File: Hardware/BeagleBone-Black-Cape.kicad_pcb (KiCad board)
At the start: 2 copper layers, 54.6 x 86.4 mm, 17 parts, among them J1 MISC, J2 POWER, J3 BOOT, J4 BOOT, M1 MR1132, M2 CC2538MODULE, P8 BeagleBone_Black_Header, P9 BeagleBone_Black_Header, Q1 2N7002, U1 MAX3072E

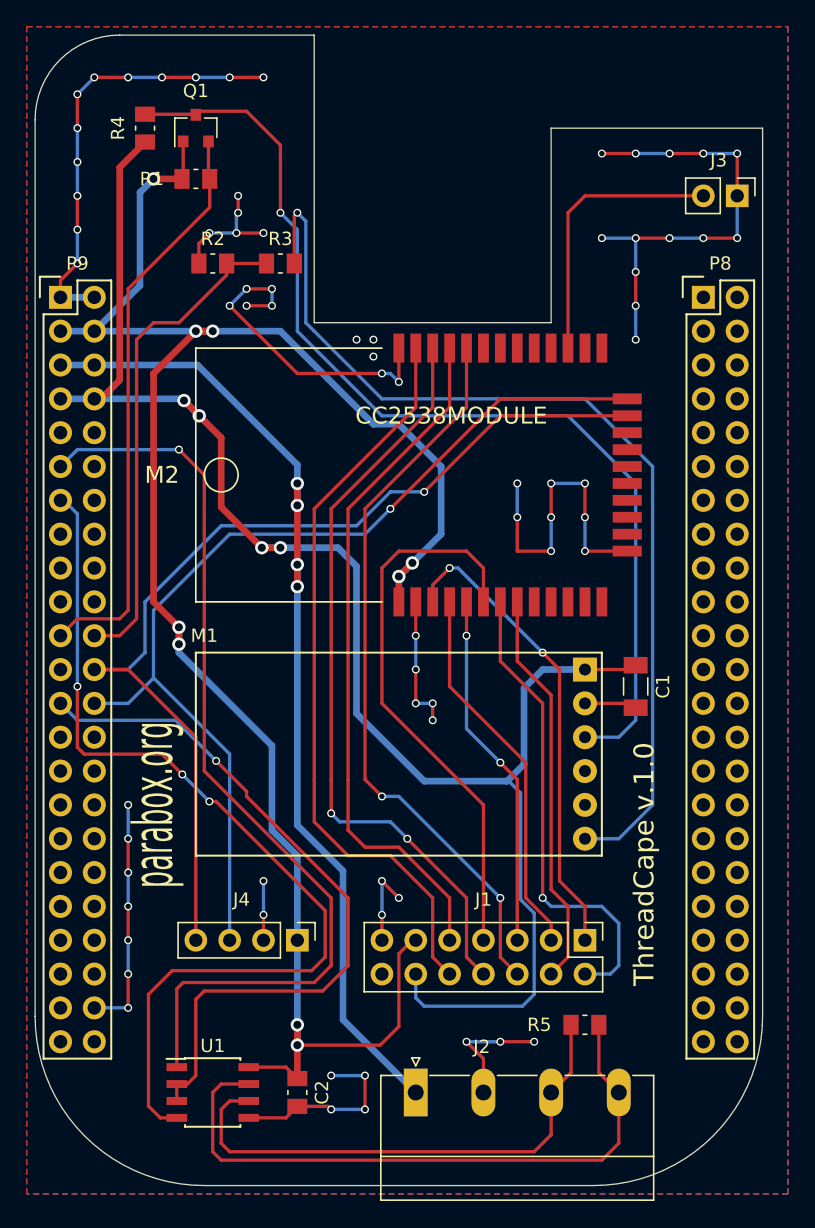
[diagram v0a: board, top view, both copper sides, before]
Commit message: Final version
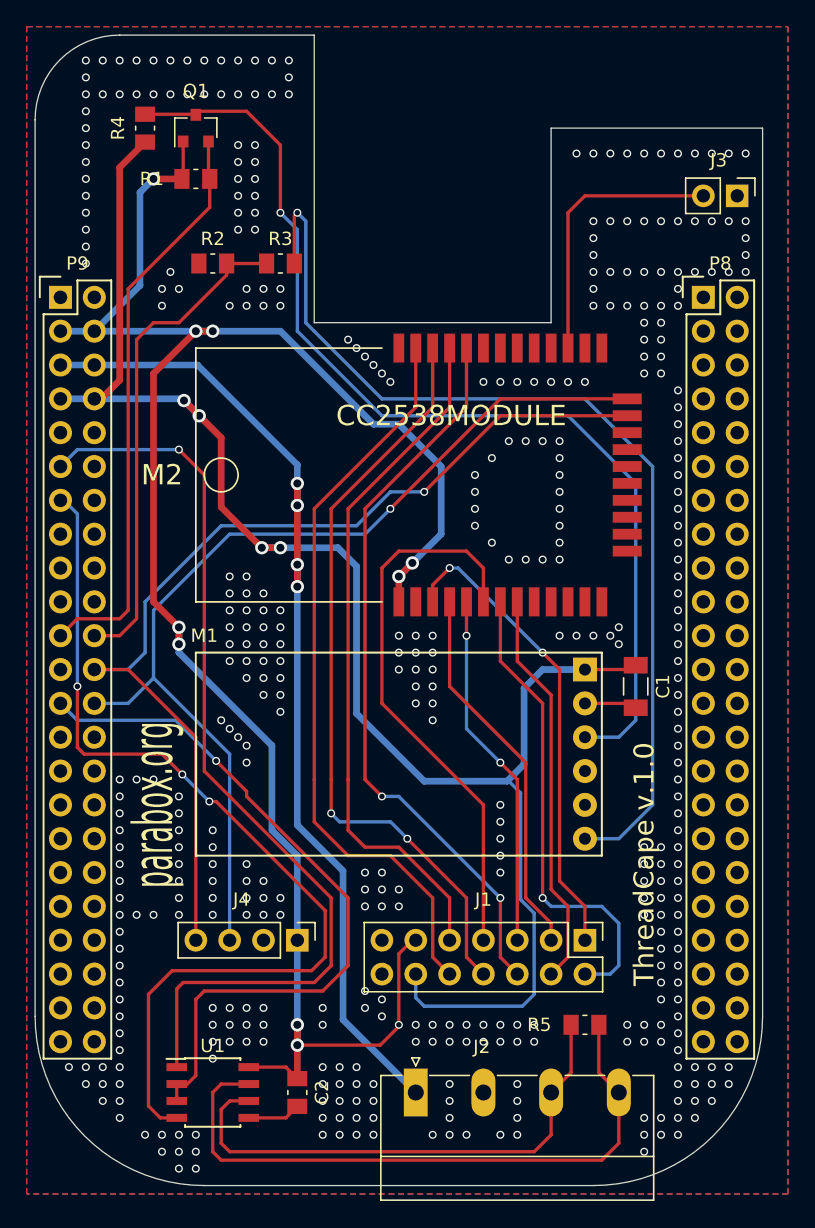
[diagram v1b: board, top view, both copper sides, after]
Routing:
- net GNDD: track 190.8 -> 7.95 mm, vias 69 -> 418
- net +3V3: vias 9 -> 10
- net (no net): vias 3 -> 0
